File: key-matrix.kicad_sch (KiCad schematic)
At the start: 138 parts, among them J1 Conn_01x12_Pin, J2 Conn_01x12_Pin, SW1 SW_Push, SW10 SW_Push, SW11 SW_Push, SW12 SW_Push, SW13 SW_Push, SW14 SW_Push, SW15 SW_Push, SW16 SW_Push, SW17 SW_Push, SW18 SW_Push, SW19 SW_Push, SW2 SW_Push, SW20 SW_Push, SW21 SW_Push, SW22 SW_Push, SW23 SW_Push, SW24 SW_Push, SW25 SW_Push, SW26 SW_Push, SW27 SW_Push, SW28 SW_Push, SW29 SW_Push, SW3 SW_Push, SW30 SW_Push, SW31 SW_Push, SW32 SW_Push, SW33 SW_Push, SW34 SW_Push, SW35 SW_Push, SW36 SW_Push, SW37 SW_Push, SW38 SW_Push, SW39 SW_Push, SW4 SW_Push, SW40 SW_Push, SW41 SW_Push, SW42 SW_Push, SW43 SW_Push, SW44 SW_Push, SW45 SW_Push, SW46 SW_Push, SW47 SW_Push, SW48 SW_Push, SW49 SW_Push, SW5 SW_Push, SW50 SW_Push, SW51 SW_Push, SW52 SW_Push, SW53 SW_Push, SW54 SW_Push, SW55 SW_Push, SW56 SW_Push, SW57 SW_Push, SW58 SW_Push, SW59 SW_Push, SW6 SW_Push, SW60 SW_Push, SW61 SW_Push, SW62 SW_Push, SW63 SW_Push, SW64 SW_Push, SW65 SW_Push, SW66 SW_Push, SW67 SW_Push, SW68 SW_Push, SW7 SW_Push, SW8 SW_Push, SW9 SW_Push

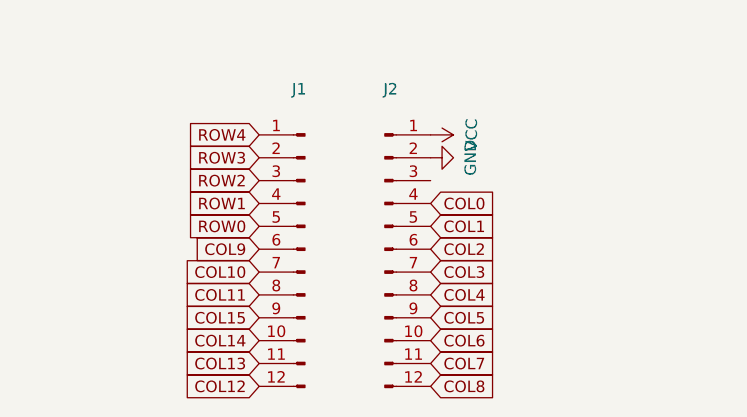
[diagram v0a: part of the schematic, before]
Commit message: checkpoint w gemini routed
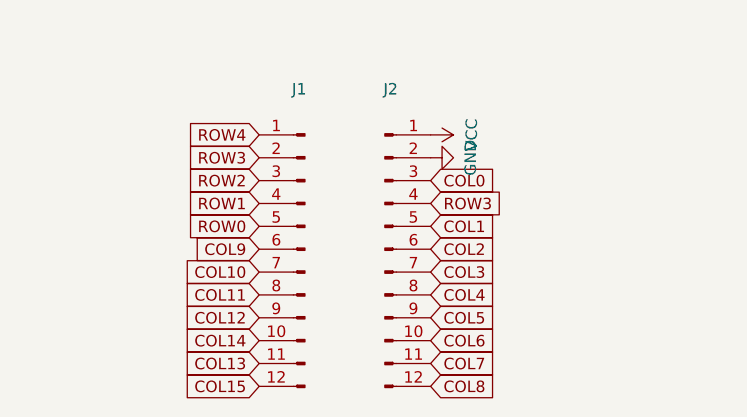
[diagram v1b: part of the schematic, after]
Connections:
- net COL0: now also J2.3 (Pin_3); no longer J2.4 (Pin_4)
- net COL12: now also J1.9 (Pin_9); no longer J1.12 (Pin_12)
- net COL15: now also J1.12 (Pin_12); no longer J1.9 (Pin_9)
- net ROW3: now also J2.4 (Pin_4)
